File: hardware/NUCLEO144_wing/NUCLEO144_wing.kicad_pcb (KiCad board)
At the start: 4 copper layers, 0 parts

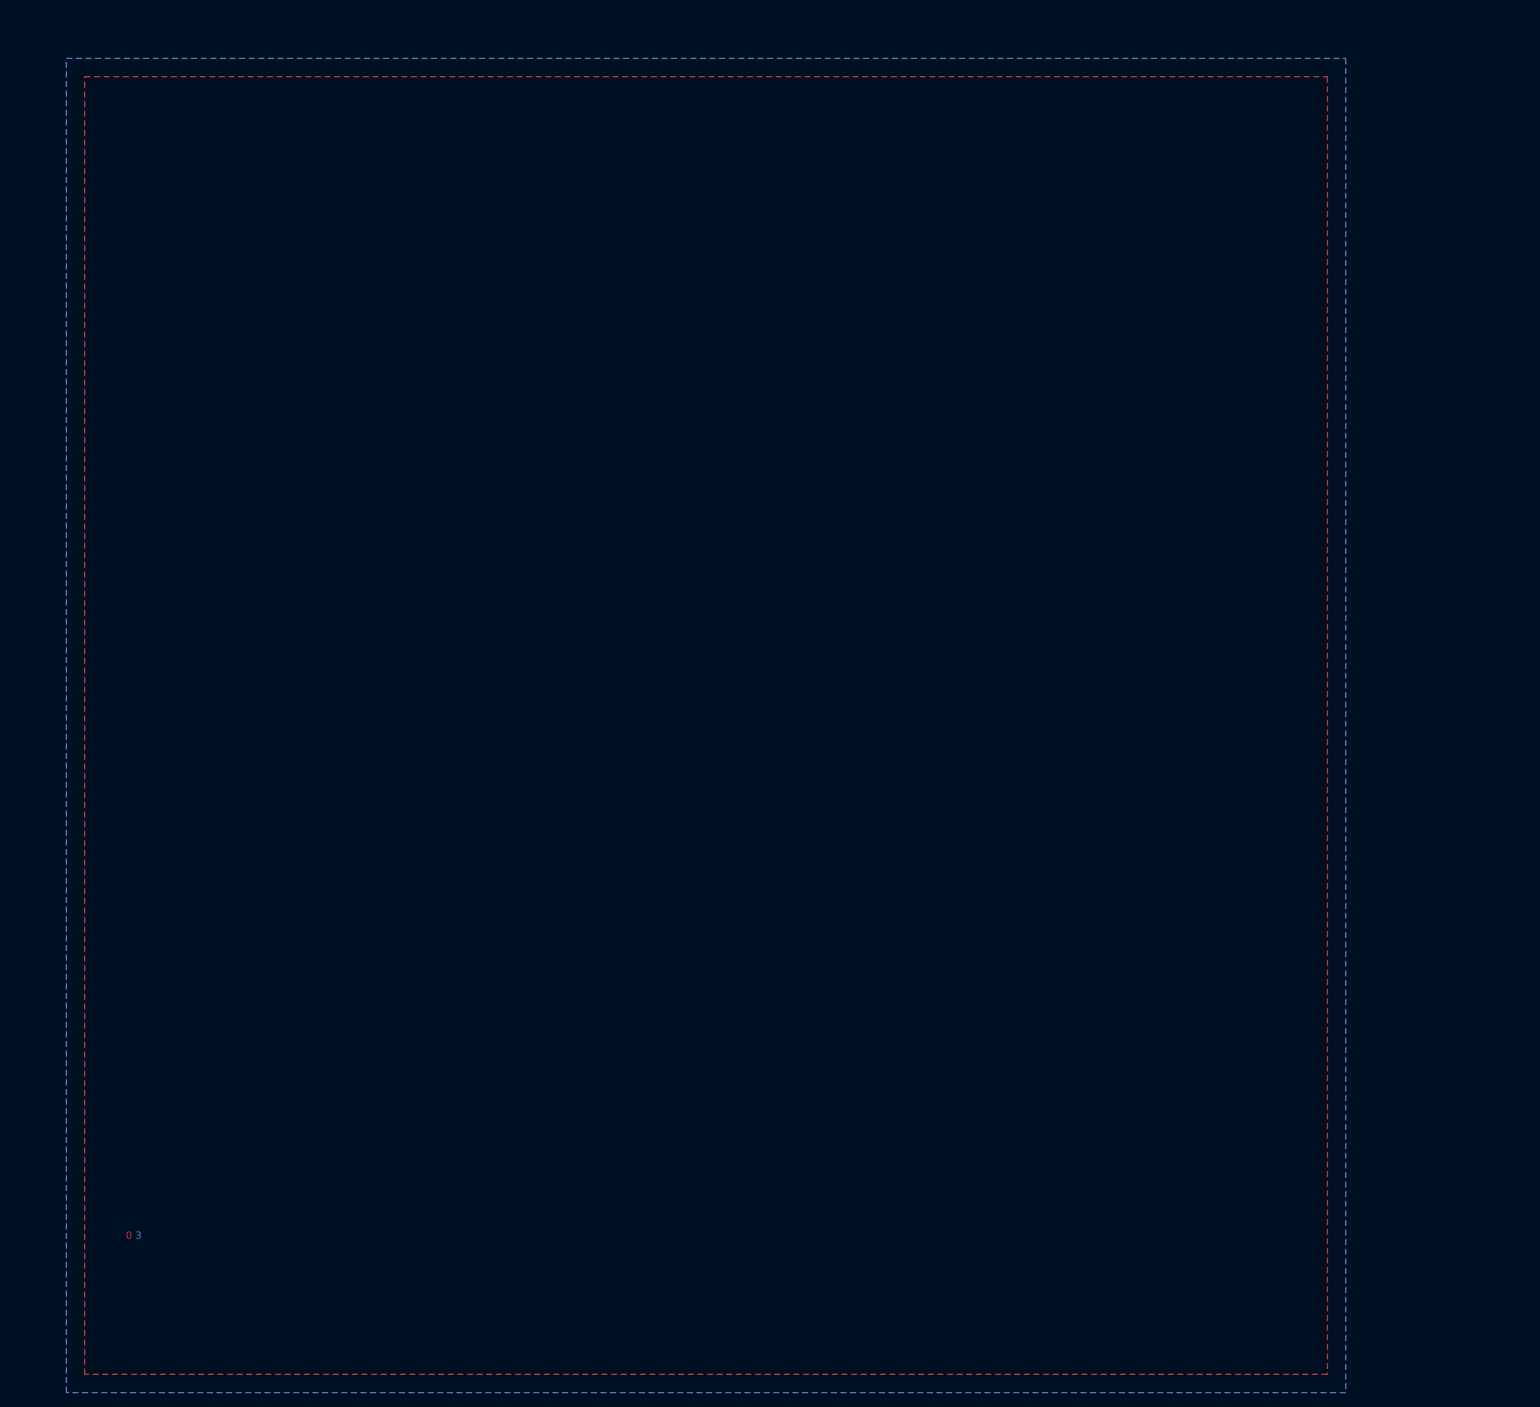
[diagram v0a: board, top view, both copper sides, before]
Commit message: p
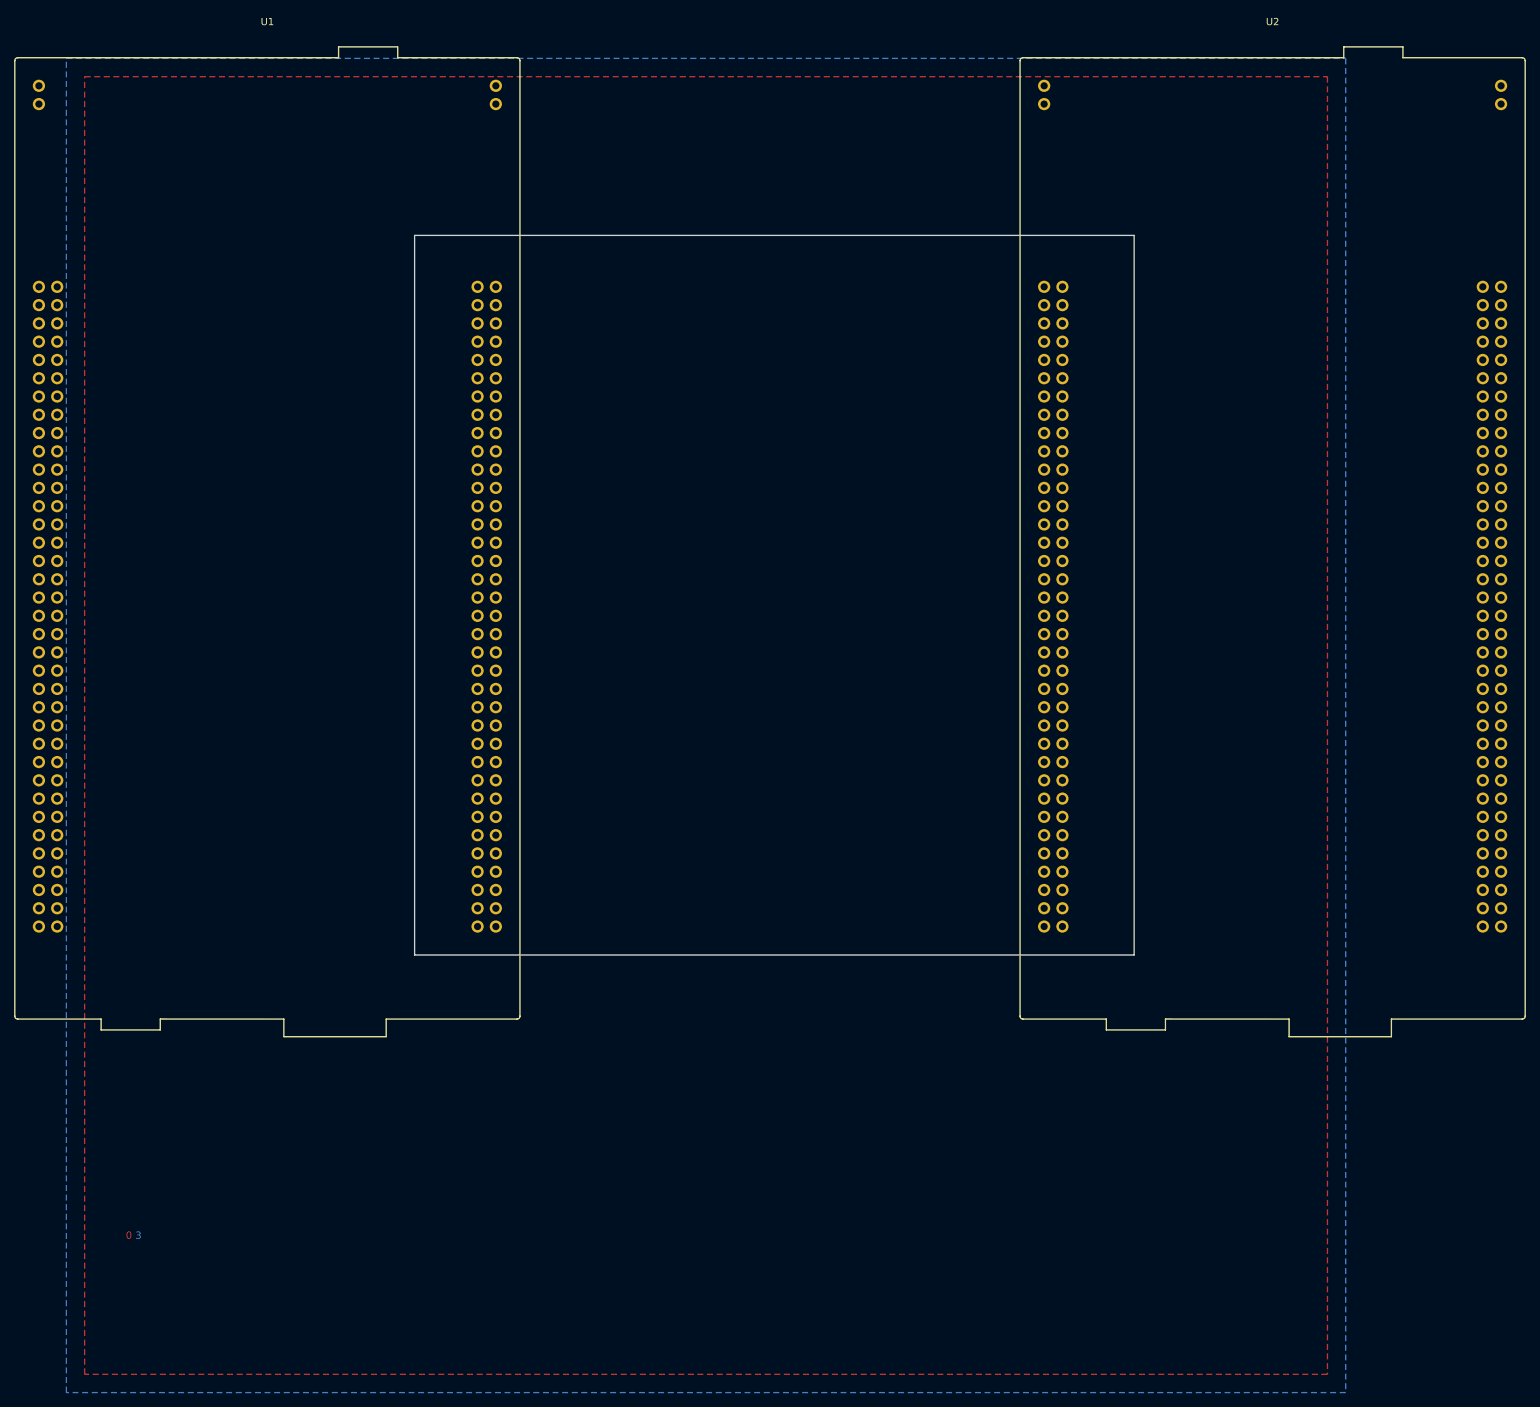
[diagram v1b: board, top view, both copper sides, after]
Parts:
- added U1: NUCLEO144-F429ZI, rusEFI_LIB:ST_Morpho_Connector_144_STLink, F.Cu at (97.8, 57.1)
- added U2: NUCLEO144-F429ZI, rusEFI_LIB:ST_Morpho_Connector_144_STLink, F.Cu at (237.5, 57.1)
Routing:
- removed copper zone on PWR, net /5V
- removed copper zone on GND, net GND
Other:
- board outline added: 100 x 100 mm
- copper layers 4 -> 2
- board text added: "2 layer board stackup is as follows: 0 is top min 1 oz copper (1.4 mil) min 47 mil core FR4 3 is bottom min 1 oz copper (1.4 mil)"
- board text removed: "4 layer board stackup is as follows: 0 is top min 1 oz copper (1.4 mil) min 6.7 mil prepreg FR4 1 is GND min 0.5 oz copper (0.7 mil) min 47 mil core FR4 2 is PWR min 0.5 oz copper (0.7 mil) min 6.7 mil prepreg FR4 3 is bottom min 1 oz copper (1.4 mil)"
